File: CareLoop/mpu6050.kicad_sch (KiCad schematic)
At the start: 6 parts, among them U3 MPU-6050

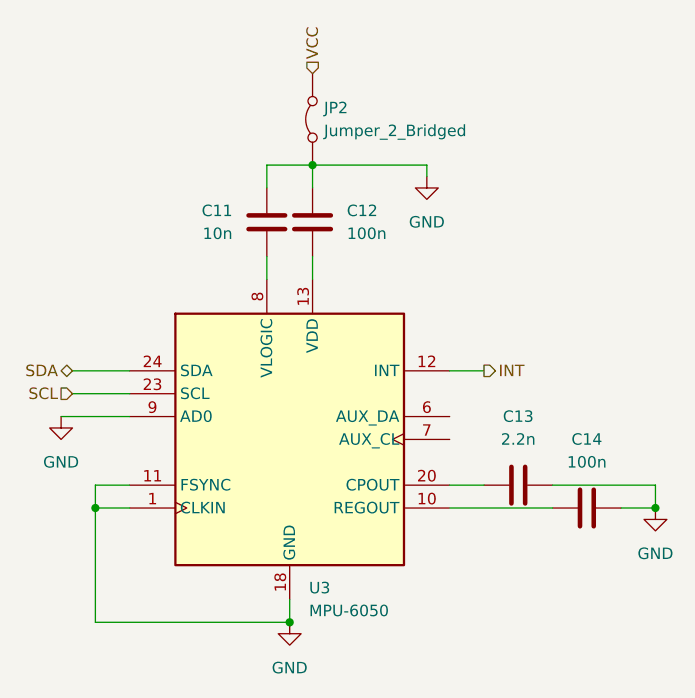
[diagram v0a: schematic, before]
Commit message: updated version
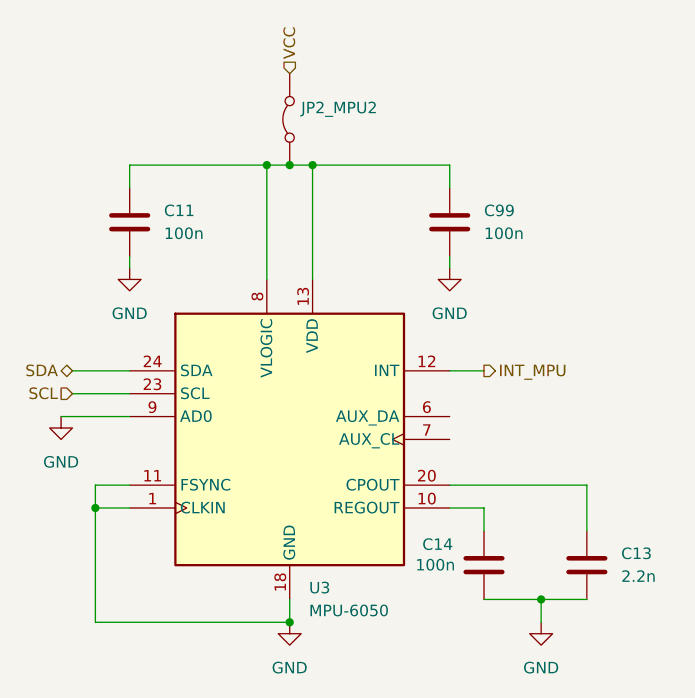
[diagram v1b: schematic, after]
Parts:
- C11: value 10n -> 100n
- renumbered C12 to C99, JP2 to JP2_MPU2
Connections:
- net GND: now also C11.1, C13.1, C99.1; no longer C11.2, C13.2, C99.2, JP2_MPU2.1 (A)
- net at U3.13 (VDD): now also C11.2, C99.2, JP2_MPU2.1 (A), U3.8 (VLOGIC); no longer C99.1
- net at U3.20 (CPOUT): now also C13.2; no longer C13.1
- net INT renamed INT_MPU
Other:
- moved on the sheet: C11, C13, C14, C99, JP2_MPU2
